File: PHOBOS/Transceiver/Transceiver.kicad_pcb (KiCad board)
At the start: 2 copper layers, 18 parts, among them J1 Conn_01x06, J2 Conn_Coaxial, U1 SX1280IMLTRT, Y1 C1E-52.000-10-1012-X-M

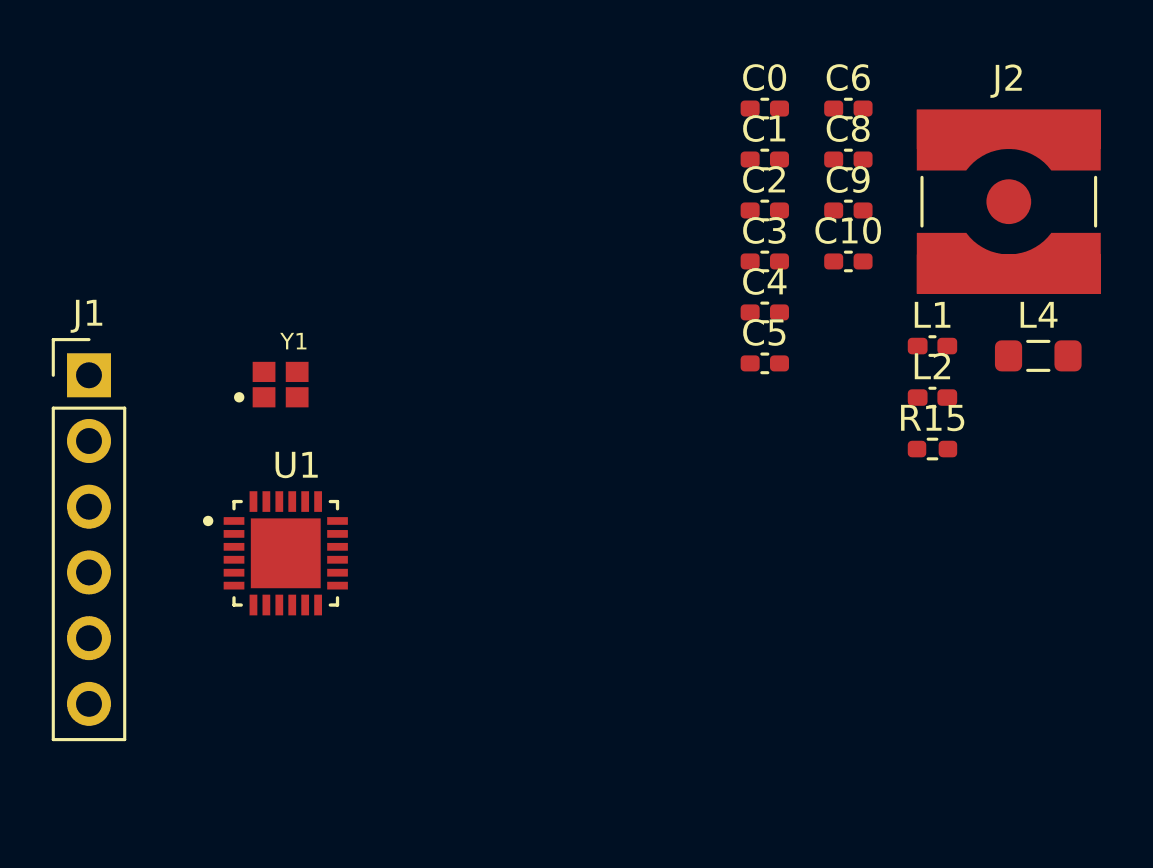
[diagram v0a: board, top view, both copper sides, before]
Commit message: Initial PCB layout updated.
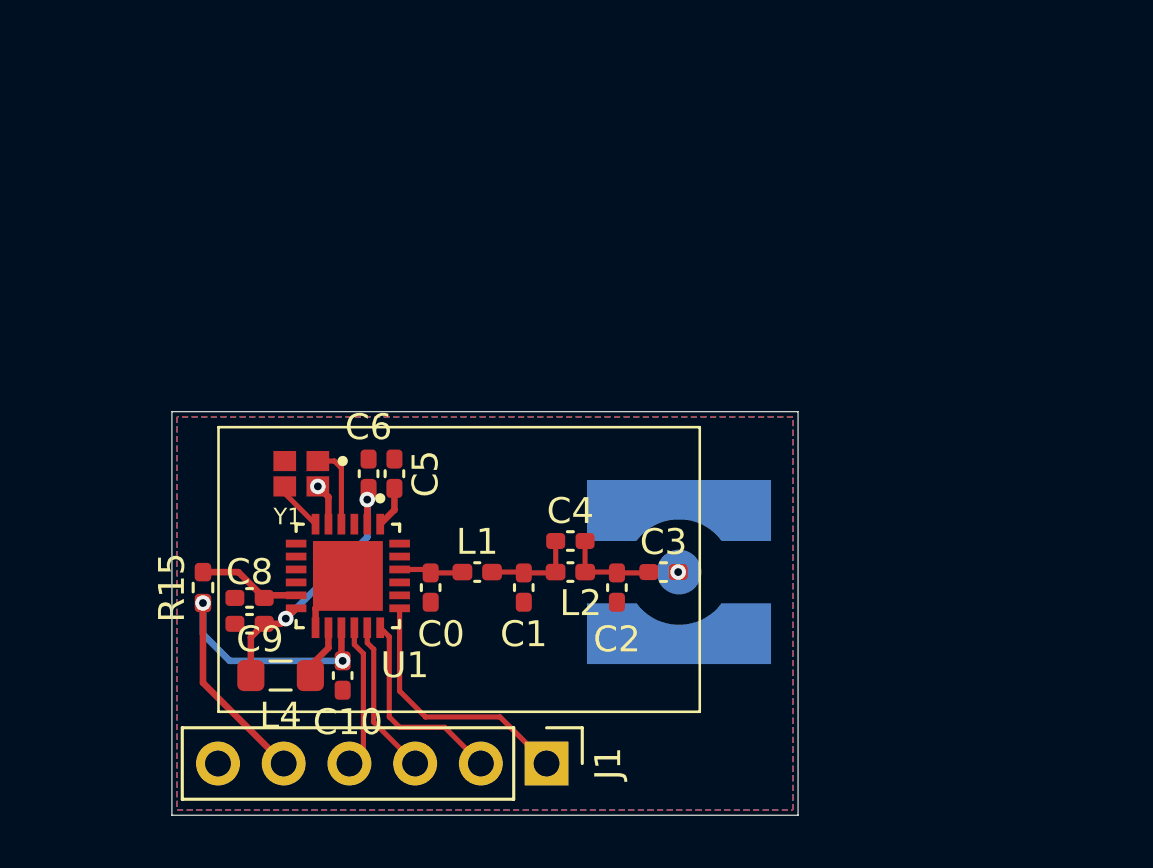
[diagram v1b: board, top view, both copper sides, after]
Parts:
- J2: moved to B.Cu
- moved L4 31.8 mm to (143.6, 97.8), turned to 180 degrees
- moved R15 28.7 mm to (140.6, 94.4), turned to -90 degrees
- moved C8 28.7 mm to (142.4, 94.8), turned to 180 degrees
- moved C9 28.1 mm to (142.4, 95.8), turned to 180 degrees
- moved C10 25.3 mm to (146.0, 97.8), turned to -90 degrees
- moved C6 23.3 mm to (147.0, 90.0), turned to 90 degrees
- moved J1 23.2 mm to (153.9, 101.2), turned to -90 degrees
- moved C0 22.6 mm to (149.4, 94.4), turned to -90 degrees
- moved L1 19.6 mm to (151.2, 93.8)
- moved J2 19.2 mm to (159.0, 93.8), turned to 180 degrees
- moved C1 19.0 mm to (153.0, 94.4), turned to -90 degrees
- moved C2 15.7 mm to (156.6, 94.4), turned to -90 degrees
- moved L2 15.5 mm to (154.8, 93.8)
- moved C5 14.9 mm to (148.0, 90.0), turned to 90 degrees
- moved C3 12.6 mm to (158.4, 93.8)
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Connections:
- net Net-(J2-In) renamed /ANTENNA
- net Net-(U1-DCC_FB) renamed /DCC_FB
- net Net-(U1-DCC_SW) renamed /DCC_SW
- net Net-(U1-RFIO) renamed /RFIO
- net Net-(U1-VBAT_IO) renamed /VBAT_IO
- net Net-(U1-VR_PA) renamed /VR_PA
- net Net-(U1-XTA) renamed /XTA
- net Net-(U1-XTB) renamed /XTB
- C10 pad 1: Net-(U1-VBAT) -> VDD
- J1 pad 1: VDD -> /NSS
- J1 pad 5: /NSS -> VDD
- U1 pad 15: Net-(U1-VBAT) -> VDD
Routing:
- net VDD: track 0.00 -> 15.8 mm, vias 0 -> 2
- net /DCC_FB: track 0.00 -> 11.0 mm, vias 0 -> 2
- net /NSS: track 0.00 -> 10.0 mm
- net /SCK: track 0.00 -> 7.88 mm
- net /MOSI: track 0.00 -> 6.02 mm
- net /MISO: track 0.00 -> 5.62 mm
- net GND: track 0.00 -> 4.15 mm, vias 0 -> 1
- net /VBAT_IO: track 0.00 -> 4.05 mm
- net Net-(C2-Pad1): track 0.00 -> 3.69 mm
- net Net-(C1-Pad1): track 0.00 -> 3.68 mm
- net /XTA: track 0.00 -> 3.19 mm
- net /RFIO: track 0.00 -> 2.50 mm
- net /DCC_SW: track 0.00 -> 2.14 mm
- net /XTB: track 0.00 -> 1.95 mm
- net /VR_PA: track 0.00 -> 1.61 mm
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- added copper zone on B.Cu, net GND
- added copper zone on F.Cu, net GND
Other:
- board outline added: 24.2 x 15.6 mm
